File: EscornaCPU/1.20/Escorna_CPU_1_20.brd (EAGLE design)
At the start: 49.9 x 89.6 mm, 97 parts, among them IC1 ULN2803, J1 2.54, U2 ESP01, U6 1117-3.3, X1 AK550/2, X1.1 AK550/2

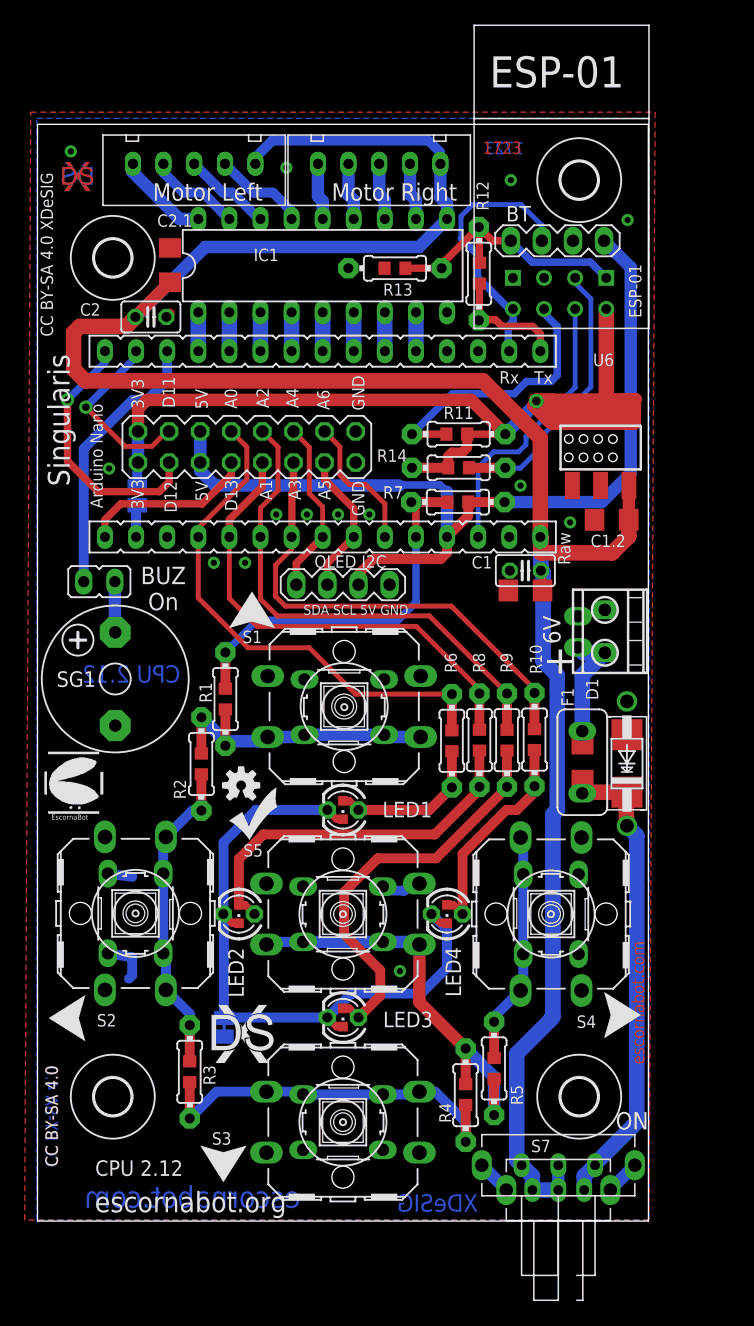
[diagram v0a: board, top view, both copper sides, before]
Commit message: New design
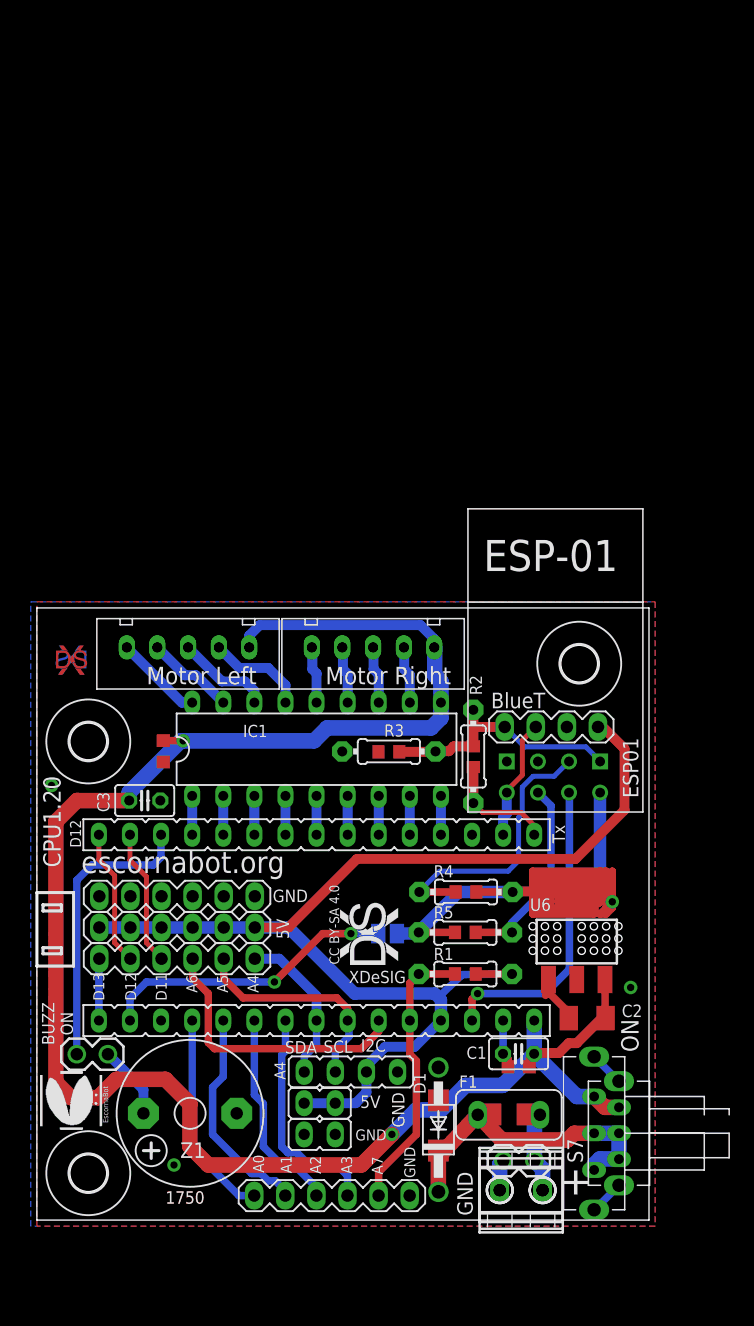
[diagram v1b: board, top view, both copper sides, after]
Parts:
- removed C1.2: 1uF, rcl:C1206
- removed C2.1: 100nF, rcl:C1206
- removed D2: K7, adafruit:SMADIODE
- removed H1, H2: MOUNT-HOLE3.0, holes:3,0
- removed J1: 2.54, con-molex:6410-02
- removed LED1, LED2, LED3, LED4: (no value), adafruit:LED3MM
- removed LED1.1, LED2.1, LED3.1, LED4.1: (no value), adafruit:CHIPLED_0603
- removed LOGO1: OSHW-LOGOS, SparkFun-Aesthetics:OSHW-LOGO-S
- removed R10, R6, R8, R9: 1K, rcl:0204/7
- removed R10.1, R6.1, R8.1, R9.1: 1K, rcl:R0603
- removed R11, R12, R14, R7: 10K, rcl:0204/7
- removed R11.1, R12.1, R14.1, R7.1: 10K, rcl:R0603
- removed R13: 18K, rcl:0204/7
- removed R13.1: 18K, rcl:R0603
- removed S1, S2, S3, S4, S5: (no value), switch-omron:B3F-10XX
- removed S1.1, S2.1, S3.1, S4.1, S5.1: (no value), switch-omron:B3F-40XX
- removed SG1: F/CM12P, buzzer:F/CM12P
- removed SJ2: (no value), jumper:SJ
- removed U$10, U$2: GO, escorna:VALE
- removed U$11, U$3, U$4, U$6, U$7, U$8, U$9: FRECHA, escorna:FRECHA
- removed U$12: XDESIG_XDESIG21, Escorna_CPU_2_01:XDESIG_XDESIG
- removed U$5: ESCORNABOT, escorna:ESCORNA_PEQUE
- added C3: 100nF, rcl:C025-025X050
- added C3.1: 100nF, rcl:C0603K
- added D1.1: M7, diode:SMA-DO214AC
- added ESC1, ESC2: ESCORNABOT, escorna:ESCORNA_PEQUE
- added H7: MOUNT-HOLE3.0, holes:3,0
- added JP2: (no value), SparkFunEagle-6-6-07:1X02
- added JP3, JP4: (no value), jumper:JP1
- added JP5: (no value), jumper:JP4
- added LOGO2: OSHW-LOGOS, SparkFun-Aesthetics:OSHW-LOGO-S
- added SV5, SV6: (no value), con-lstb:MA06-1
- added Z1: CFG12, buzzer:F/CM12P
- C1.1: device rcl:C1206 -> rcl:C0603K
- C2: value 100nF -> 1uF; device rcl:C025-025X050 -> rcl:C1206K
- H3, H4: value MOUNT-HOLE3.0 -> H3.0
- JP1: device jumper:JP1 -> SparkFunEagle-6-6-07:1X02
- R3, R3.1: value 10K -> 18K
- R5, R5.1: value 22K -> 10K
- SV1: value (none) -> 1x15 SOCKET STRIP; device con-lstb:MA08-2 -> escorna_LBREscorna_CPU_2_10:CON-LSTA_FE15
- SV2: value (none) -> 1x15 SOCKET STRIP
- SV3: device escorna_LBREscorna_CPU_2_10:CON-LSTA_FE15 -> con-lstb:MA06-1
- SV4: device con-lstb:MA04-1 -> con-lstb:MA06-1
- U$1: value FRECHA -> XDESIG_XDESIG21; device escorna:FRECHA -> Escorna_CPU_2_01:XDESIG_XDESIG
- moved C2 67.5 mm to (45.0, 16.5), turned to 0 degrees
- moved SV3 51.0 mm to (11.4, 21.4)
- moved X1 46.2 mm to (39.6, 2.44), flipped to the top, turned to 0 degrees
- moved X1.1 46.2 mm to (39.6, 2.44), turned to 180 degrees
- moved SJ1 41.2 mm to (28.6, 23.4), turned to 0 degrees
- moved U6 40.4 mm to (44.1, 22.8)
- moved U3 39.7 mm to (42.0, 40.3)
- moved H4 39.6 mm to (4.20, 39.1)
- moved XDS 39.5 mm to (1.57, 44.6)
- moved XDS1 39.5 mm to (4.05, 44.6)
- moved IC1 39.5 mm to (22.8, 38.5)
- moved SV2 39.5 mm to (22.8, 16.3)
- moved XH1 39.5 mm to (12.2, 47.0)
- moved XH2 39.5 mm to (27.3, 47.0)
- moved XH3 39.5 mm to (12.2, 46.6)
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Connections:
- removed net K: LED1.1.C, LED1.K, LED2.1.C, LED2.K, LED3.1.C, LED3.K, LED4.1.C, LED4.K, SJ2.2
- removed net N$12: F1.1, F1.1.1, J1.1, X1.1, X1.1.1
- removed net N$14: R14.1, R14.1.1, U2.GPIO0
- removed net N$4: LED2.1.A, LED2.A, R8.1.2, R8.2
- removed net N$5: LED1.1.A, LED1.A, R6.1.2, R6.2
- removed net N$6: LED3.1.A, LED3.A, R9.1.2, R9.2
- removed net N$8: LED4.1.A, LED4.A, R10.1, R10.1.2
- removed net S1: R1.1, R1.1.1, R2.1.2, R2.2, S1.1.3, S1.1.4, S1.3, S1.4
- removed net S2: R2.1, R2.1.1, R3.1.2, R3.2, S2.1.3, S2.1.4, S2.3, S2.4
- removed net S3: R3.1, R3.1.1, R4.1.2, R4.2, S3.1.3, S3.1.4, S3.3, S3.4
- removed net S4: R5.1, R5.1.1, S4.1.3, S4.1.4, S4.3, S4.4
- removed net S5: R4.1, R4.1.1, R5.1.2, R5.2, S5.1.3, S5.1.4, S5.3, S5.4
- new net N$1: R5.1.2, R5.2, U2.CH_PD
- new net VIN: D1.1.K, D1.C, F1.1.2, F1.2, S7.1.P$1, S7.1.P$3, S7.P$1, S7.P$3
- net 3V3: now also R4.1, R4.1.1, R5.1, R5.1.1; no longer R11.1, R11.1.1, R14.1.2, R14.2, SV1.15, SV1.16
- net 5V: now also JP3.1, JP3.2, JP5.3, R1.1, R1.1.1, SV4.1, SV4.2, SV4.4, SV4.5, SV4.6; no longer R7.1, R7.1.1, SV1.11, SV1.12
- net A0: now also SV6.1; no longer R6.1, R6.1.1, SV1.9
- net A1: now also SV6.2; no longer R8.1, R8.1.1, SV1.8
- net A2: now also SV6.3; no longer R9.1, R9.1.1, SV1.7
- net A3: now also SV6.4; no longer R10.1.1, R10.2, SV1.6
- net A4: now also JP5.1, SV3.1; no longer SV1.5, SV4.1
- net A5: now also JP5.2, SV3.2; no longer SV1.4, SV4.2
- net A6: now also SV3.3; no longer SV1.3
- net A7: now also SV6.5; no longer R7.1.2, R7.2
- net CH: now also R4.1.2, R4.2, U2.GPIO0; no longer R11.1.2, R11.2, U2.CH_PD
- net D10: now also SV1.13; no longer SV3.13
- net D11: now also SV1.14, SV3.4; no longer SV1.13, SV3.14
- net D12: now also SV1.15, SV3.5; no longer SV1.14, SV3.15
- net D13: now also SV3.6; no longer SV1.10
- net D2: now also SV1.5; no longer SV3.5
- net D3: now also SV1.6; no longer SV3.6
- net D4: now also SV1.7; no longer SV3.7
- net D5: now also SV1.8; no longer SV3.8
- net D6: now also SV1.9; no longer SV3.9
- net D7: now also SV1.10; no longer SV3.10
- net D8: now also SV1.11; no longer SV3.11
- net D9: now also SV1.12; no longer SV3.12
- net GND: now also C1.2, C3.1, C3.1.1, D1.1.A, JP2.1, JP4.1, JP4.2, JP5.4, R3.1.1, R3.2, SV1.4, SV5.1, SV5.2, SV5.3, SV5.4, SV5.5, SV5.6, SV6.6, X1.1, Z1.-; no longer C1.1, C1.2.1, C2.1.1, D2.A, J1.2, R13.1.1, R13.2, S1.1, S1.1.1, S1.1.2, S1.2, S2.1, S2.1.1, S2.1.2, S2.2, S3.1, S3.1.1, S3.1.2, S3.2, S4.1, S4.1.1, S4.1.2, S4.2, S5.1, S5.1.1, S5.1.2, S5.2, SG1.-, SJ2.1, SV1.1, SV1.2, SV3.4, SV4.4, X1.2
- net N$2: now also Z1.+; no longer SG1.+
- net N$3: now also F1.1, F1.1.1, JP2.2, X1.1.1, X1.2; no longer D1.C, D2.C, F1.1.2, F1.2, S7.1.P$2, S7.P$2
- net RAW: now also C1.1, C3.1.2, C3.2, S7.1.P$2, S7.P$2; no longer C1.2, C1.2.2, C2.1.2, S7.1.P$1, S7.1.P$3, S7.P$1, S7.P$3
- net RX: now also SV1.2; no longer SV3.2
- net TX: now also R2.1, R2.1.1, SV1.1; no longer R12.1, R12.1.1, SV3.1
- net TX3V3: now also R2.1.2, R2.2, R3.1, R3.1.2; no longer R12.1.2, R12.2, R13.1, R13.1.2
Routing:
- net K: track 55.1 -> 0.00 mm
- net S5: track 35.0 -> 0.00 mm
- net RAW: track 188.7 -> 153.8 mm, vias 0 -> 2
- net N$6: track 33.6 -> 0.00 mm
- net S3: track 32.2 -> 0.00 mm
- net N$3: track 39.4 -> 7.83 mm
- net N$4: track 30.6 -> 0.00 mm
- net 3V3: track 112.7 -> 84.6 mm
- net VIN: track 0.00 -> 26.6 mm
- net S2: track 26.1 -> 0.00 mm
- net A0: track 42.7 -> 17.1 mm
- net S1: track 25.2 -> 0.00 mm
- net A2: track 41.1 -> 17.0 mm
- net 5V: track 76.1 -> 99.2 mm
- net N$14: track 22.7 -> 0.00 mm
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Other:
- board size 49.9 x 89.6 mm -> 50 x 50 mm
- board text added: "1750"
- board text added: "A7"
- board text added: "BUZZ ON"
- board text added: "BlueT"
- board text added: "CPU1.20"
- board text added: "ESP01"
- board text added: "Escorna_CPU V1.20"
- board text added: "I2C"
- board text added: "SCL"
- board text added: "SDA"
- board text added: "Sel 3V3"
- board text removed: "1723"
- board text removed: "3V3"
- board text removed: "3V3 select"
- board text removed: "6V"
- board text removed: "Arduino Nano"
- board text removed: "BT"
- board text removed: "BUZ On"
- board text removed: "C2.1"
- board text removed: "CC BY-SA 4.0 XDeSIG"
- board text removed: "CPU 2.12"
- board text removed: "ESP-01"
- board text removed: "Expansion"
- board text removed: "L-on"
- board text removed: "OLED I2C"
- board text removed: "Raw"
- board text removed: "Rx"
- board text removed: "SDA SCL 5V GND"
- board text removed: "Singularis"
- board text removed: "connector"
- board text removed: "http://escornabot.org"
